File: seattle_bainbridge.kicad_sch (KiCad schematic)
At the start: 17 parts

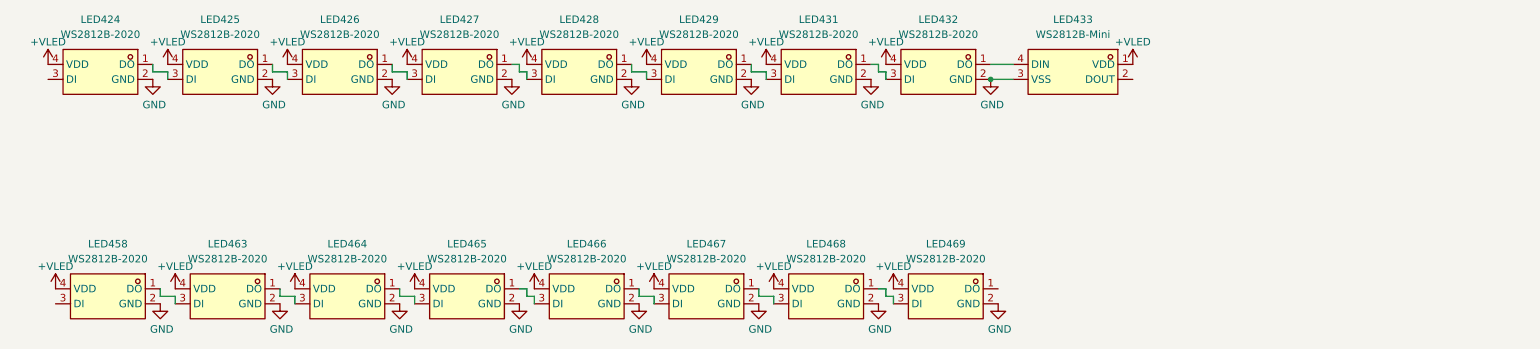
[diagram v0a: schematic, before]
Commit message: single ferry track checkpoint
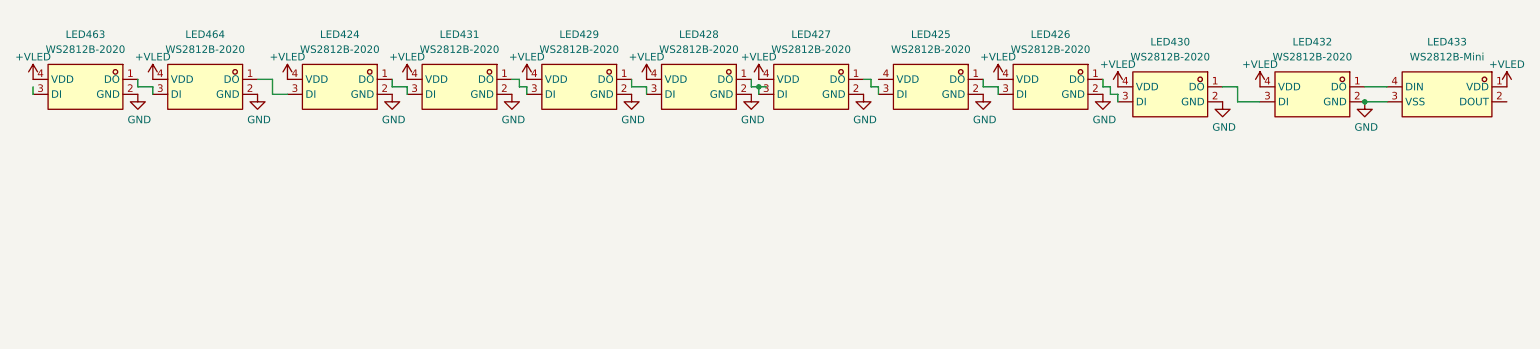
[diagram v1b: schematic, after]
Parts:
- removed LED458, LED465, LED466, LED467, LED468, LED469: WS2812B-2020, EasyEDA:LED-SMD_4P-L2.0-W2.0-TL_WS2812B-2020, symbol EasyEDA:WS2812B-2020
- added LED430: WS2812B-2020, EasyEDA:LED-SMD_4P-L2.0-W2.0-TL_WS2812B-2020, symbol EasyEDA:WS2812B-2020
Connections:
- net +VLED: now also LED430.4 (VDD); no longer LED425.4 (VDD)
- net GND: now also LED430.2 (GND)
- net at LED464.1 (DO): now also LED424.3 (DI)
- net at LED431.3 (DI): now also LED424.1 (DO); no longer LED429.1 (DO)
- net at LED429.3 (DI): now also LED431.1 (DO); no longer LED428.1 (DO)
- net at LED427.1 (DO): now also LED425.3 (DI); no longer LED428.3 (DI)
- net at LED426.1 (DO): now also LED430.3 (DI); no longer LED427.3 (DI)
- net at LED432.3 (DI): now also LED430.1 (DO); no longer LED431.1 (DO)
- new net: LED427.3 (DI), LED428.1 (DO)
- new net: LED428.3 (DI), LED429.1 (DO)
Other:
- moved on the sheet: LED424, LED463, LED464
